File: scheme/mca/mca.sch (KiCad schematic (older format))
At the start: 1 part

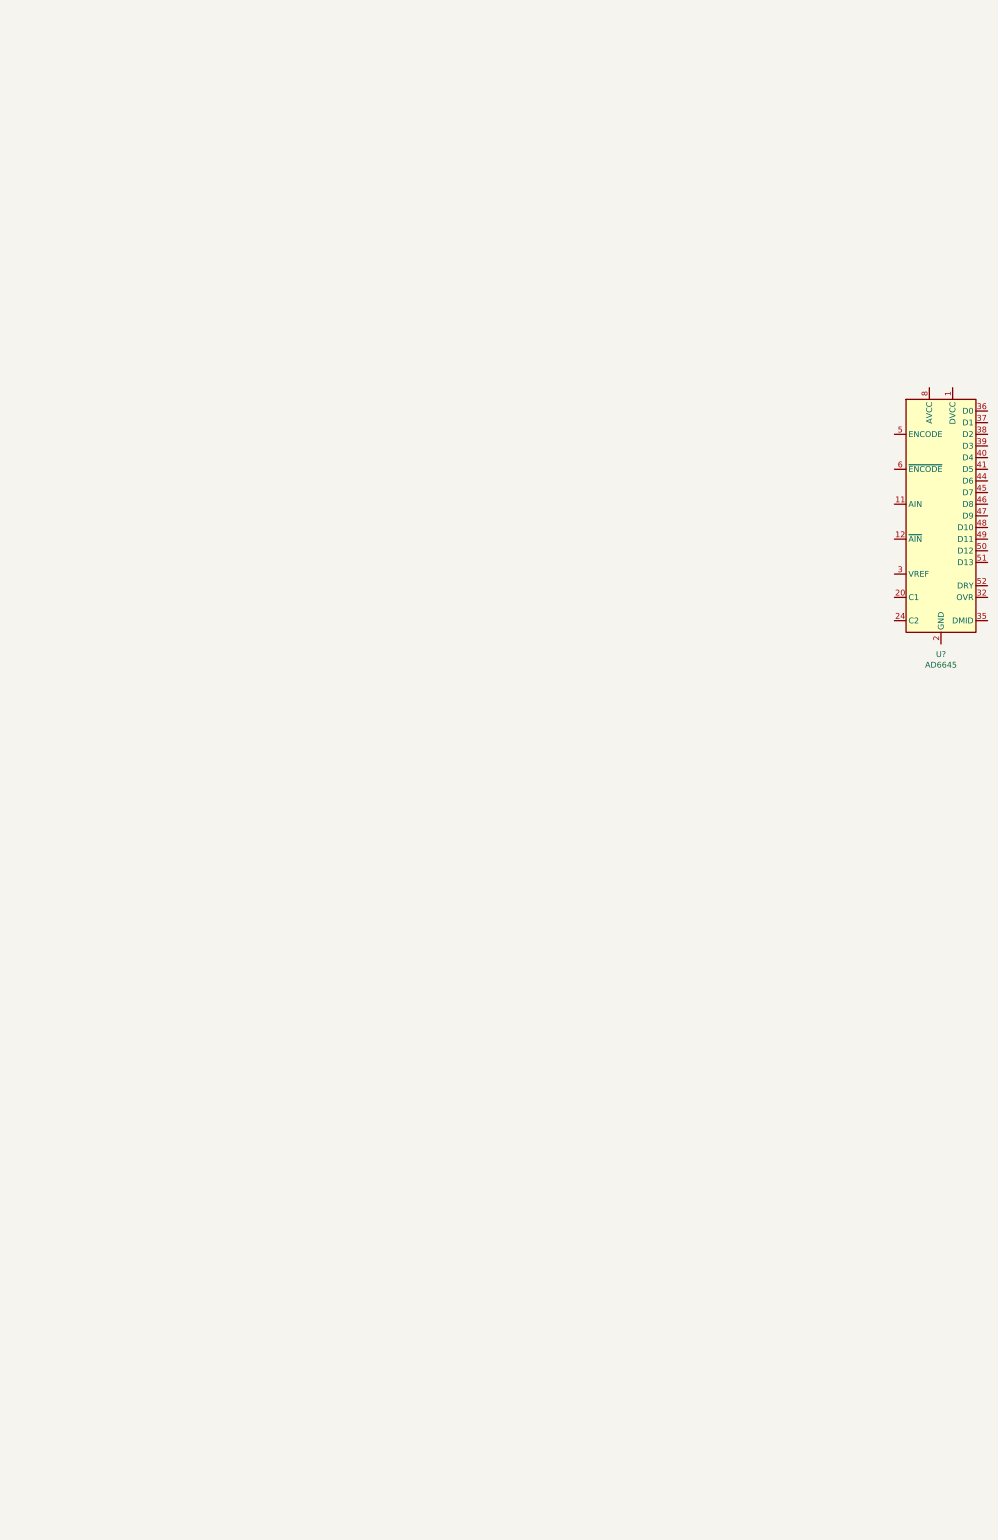
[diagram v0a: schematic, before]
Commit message: +start work on scheme
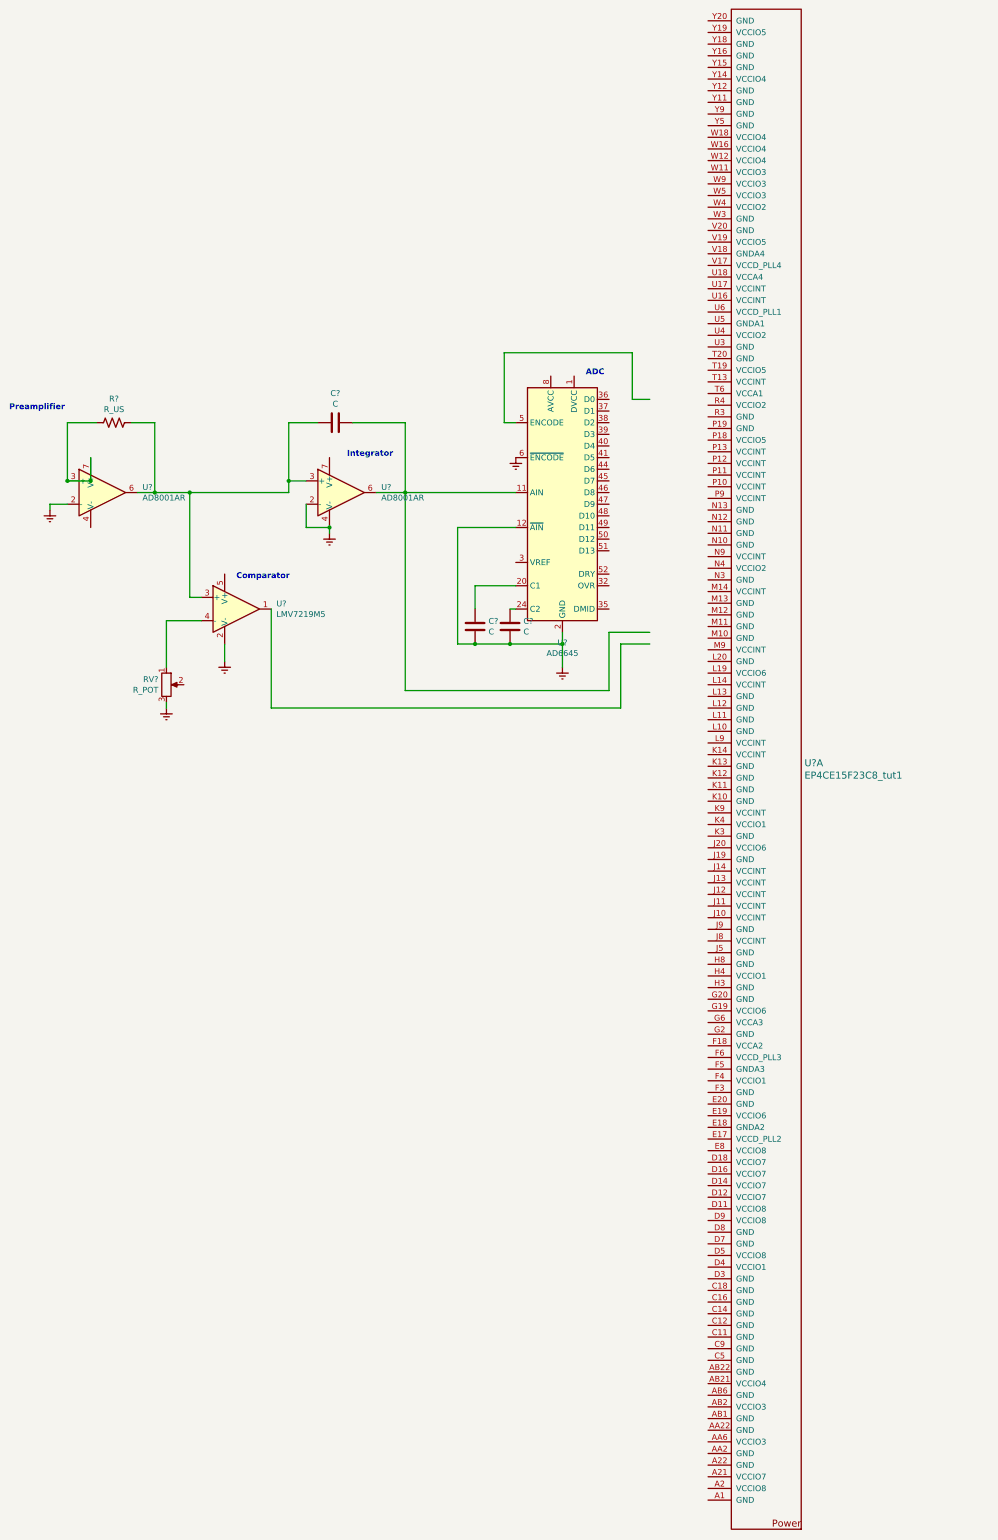
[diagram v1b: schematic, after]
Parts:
- added C? (x3): C, symbol Device:C
- added R?: R_US, symbol Device:R_US
- added RV?: R_POT, symbol Device:R_POT
- added U?: LMV7219M5, Package_TO_SOT_SMD:SOT-23-5, symbol Comparator:LMV7219M5
- added U? (x2): AD8001AR, Package_SO:SOIC-8_3.9x4.9mm_P1.27mm, symbol Amplifier_Operational:AD8001AR
- added U?: EP4CE15F23C8_tut1, Package_QFP:LQFP-144_20x20mm_P0.5mm, symbol ep4ce15:EP4CE15F23C8_tut1
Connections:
- net labels added: Earth
- wire segments 0 -> 51
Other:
- note added: "ADC"
- note added: "Comparator"
- note added: "Integrator"
- note added: "Preamplifier"
- moved on the sheet: U?
